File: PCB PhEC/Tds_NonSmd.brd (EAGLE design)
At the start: 194.3 x 107.6 mm, 61 parts, among them IC1 TL074P, IC2 TL062P, X10 227161-8, X2 BN35N61, X4 R141426, X5 R141426, X8 BN35N61, X9 227161-8

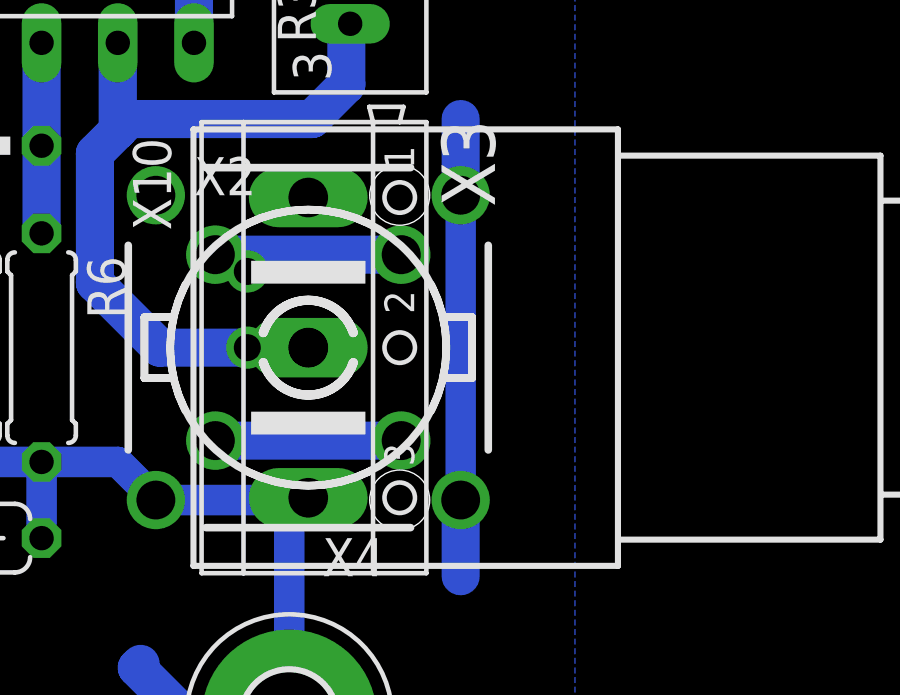
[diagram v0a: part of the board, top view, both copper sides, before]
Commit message: ADD PCB READY TO PRINT
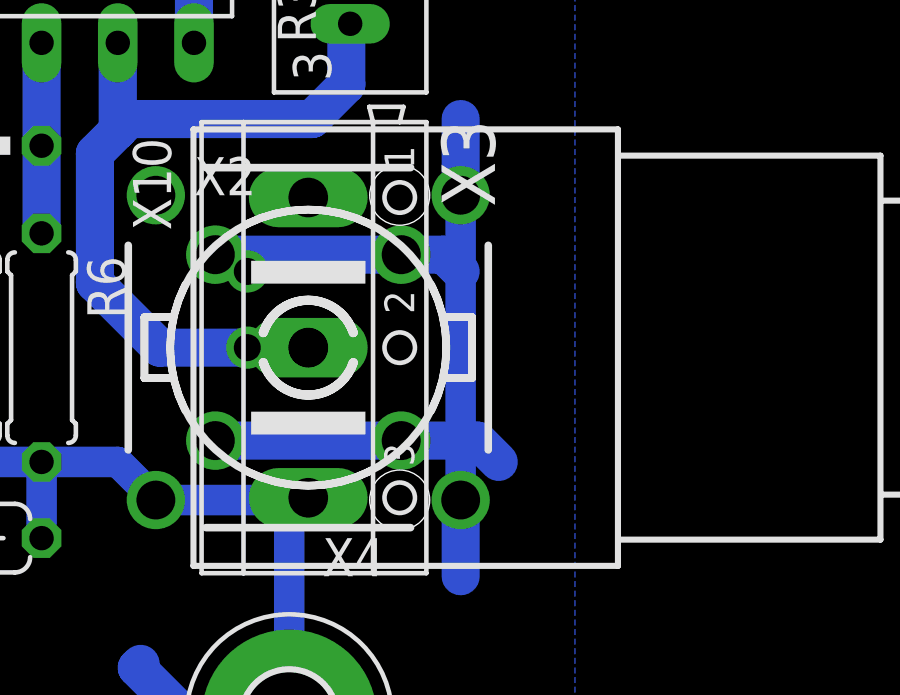
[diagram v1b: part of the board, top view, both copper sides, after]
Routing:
- net AGND: track 278.2 -> 283.9 mm
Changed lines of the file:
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@@
 <grid distance="50" unitdist="mil" unit="mm" style="lines" multiple="1" display="yes" altdistance="5" altunitdist="mil" altunit="mm"/>
 <layers>
-<layer number="1" name="Top" color="4" fill="1" visible="yes" active="yes"/>
+<layer number="1" name="Top" color="4" fill="1" visible="no" active="yes"/>
 <layer number="2" name="Route2" color="16" fill="1" visible="no" active="no"/>
 <layer number="3" name="Route3" color="17" fill="1" visible="no" active="no"/>
@@
 <layer number="19" name="Unrouted" color="6" fill="1" visible="yes" active="yes"/>
 <layer number="20" name="Dimension" color="24" fill="1" visible="yes" active="yes"/>
-<layer number="21" name="tPlace" color="7" fill="1" visible="yes" active="yes"/>
+<layer number="21" name="tPlace" color="7" fill="1" visible="no" active="yes"/>
 <layer number="22" name="bPlace" color="7" fill="1" visible="yes" active="yes"/>
-<layer number="23" name="tOrigins" color="15" fill="1" visible="yes" active="yes"/>
+<layer number="23" name="tOrigins" color="15" fill="1" visible="no" active="yes"/>
 <layer number="24" name="bOrigins" color="15" fill="1" visible="yes" active="yes"/>
-<layer number="25" name="tNames" color="7" fill="1" visible="yes" active="yes"/>
+<layer number="25" name="tNames" color="7" fill="1" visible="no" active="yes"/>
 <layer number="26" name="bNames" color="7" fill="1" visible="yes" active="yes"/>
-<layer number="27" name="tValues" color="7" fill="1" visible="yes" active="yes"/>
-<layer number="28" name="bValues" color="7" fill="1" visible="yes" active="yes"/>
+<layer number="27" name="tValues" color="7" fill="1" visible="no" active="yes"/>
+<layer number="28" name="bValues" color="7" fill="1" visible="no" active="yes"/>
 <layer number="29" name="tStop" color="7" fill="3" visible="no" active="yes"/>
 <layer number="30" name="bStop" color="7" fill="6" visible="no" active="yes"/>
@@
 <layer number="37" name="tTest" color="7" fill="1" visible="no" active="yes"/>
 <layer number="38" name="bTest" color="7" fill="1" visible="no" active="yes"/>
-<layer number="39" name="tKeepout" color="4" fill="11" visible="yes" active="yes"/>
+<layer number="39" name="tKeepout" color="4" fill="11" visible="no" active="yes"/>
 <layer number="40" name="bKeepout" color="1" fill="11" visible="yes" active="yes"/>
-<layer number="41" name="tRestrict" color="4" fill="10" visible="yes" active="yes"/>
+<layer number="41" name="tRestrict" color="4" fill="10" visible="no" active="yes"/>
 <layer number="42" name="bRestrict" color="1" fill="10" visible="yes" active="yes"/>
-<layer number="43" name="vRestrict" color="2" fill="10" visible="yes" active="yes"/>
+<layer number="43" name="vRestrict" color="2" fill="10" visible="no" active="yes"/>
 <layer number="44" name="Drills" color="7" fill="1" visible="no" active="yes"/>
-<layer number="45" name="Holes" color="7" fill="1" visible="no" active="yes"/>
+<layer number="45" name="Holes" color="7" fill="1" visible="yes" active="yes"/>
 <layer number="46" name="Milling" color="3" fill="1" visible="no" active="yes"/>
 <layer number="47" name="Measures" color="7" fill="1" visible="no" active="yes"/>
-<layer number="48" name="Document" color="7" fill="1" visible="yes" active="yes"/>
-<layer number="49" name="Reference" color="7" fill="1" visible="yes" active="yes"/>
-<layer number="51" name="tDocu" color="7" fill="1" visible="yes" active="yes"/>
+<layer number="48" name="Document" color="7" fill="1" visible="no" active="yes"/>
+<layer number="49" name="Reference" color="7" fill="1" visible="no" active="yes"/>
+<layer number="51" name="tDocu" color="7" fill="1" visible="no" active="yes"/>
 <layer number="52" name="bDocu" color="7" fill="1" visible="yes" active="yes"/>
 <layer number="88" name="SimResults" color="9" fill="1" visible="no" active="no"/>
@@
 <wire x1="39.37" y1="40.64" x2="38.1" y2="41.91" width="1.016" layer="16"/>
 <wire x1="38.1" y1="41.91" x2="35.56" y2="41.91" width="1.016" layer="16"/>
-<wire x1="49.53" y1="50.8" x2="49.53" y2="40.64" width="1.016" layer="16"/>
+<wire x1="49.53" y1="50.8" x2="49.53" y2="48.26" width="1.016" layer="16"/>
+<wire x1="49.53" y1="48.26" x2="49.53" y2="40.64" width="1.016" layer="16"/>
 <wire x1="44.45" y1="40.64" x2="39.37" y2="40.64" width="1.016" layer="16"/>
 <wire x1="35.56" y1="39.37" x2="35.56" y2="41.91" width="1.016" layer="16"/>
@@
 <wire x1="50.134540625" y1="80.040459375" x2="50.53" y2="80.43591875" width="1.27" layer="16"/>
 <wire x1="50.53" y1="80.43591875" x2="50.53" y2="81.534" width="1.27" layer="16"/>
+<wire x1="47.5488" y1="48.8188" x2="48.9712" y2="48.8188" width="1.27" layer="16"/>
+<wire x1="48.9712" y1="48.8188" x2="49.53" y2="48.26" width="1.27" layer="16"/>
+<wire x1="47.5488" y1="42.6212" x2="50.0888" y2="42.6212" width="1.27" layer="16"/>
+<wire x1="50.0888" y1="42.6212" x2="50.8" y2="41.91" width="1.27" layer="16"/>
 <wire x1="47.9298" y1="89.7128" x2="48.97708125" y2="89.043" width="0" layer="19" extent="16-16"/>
 </signal>
